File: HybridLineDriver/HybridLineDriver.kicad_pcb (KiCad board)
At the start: 2 copper layers, 100 x 50 mm, 60 parts, among them J1 XLR3, J2 Conn_01x03, J3 Conn_01x02, J4 XLR3, J5 Conn_01x02, U1 OPA1679, U2 OPA1679

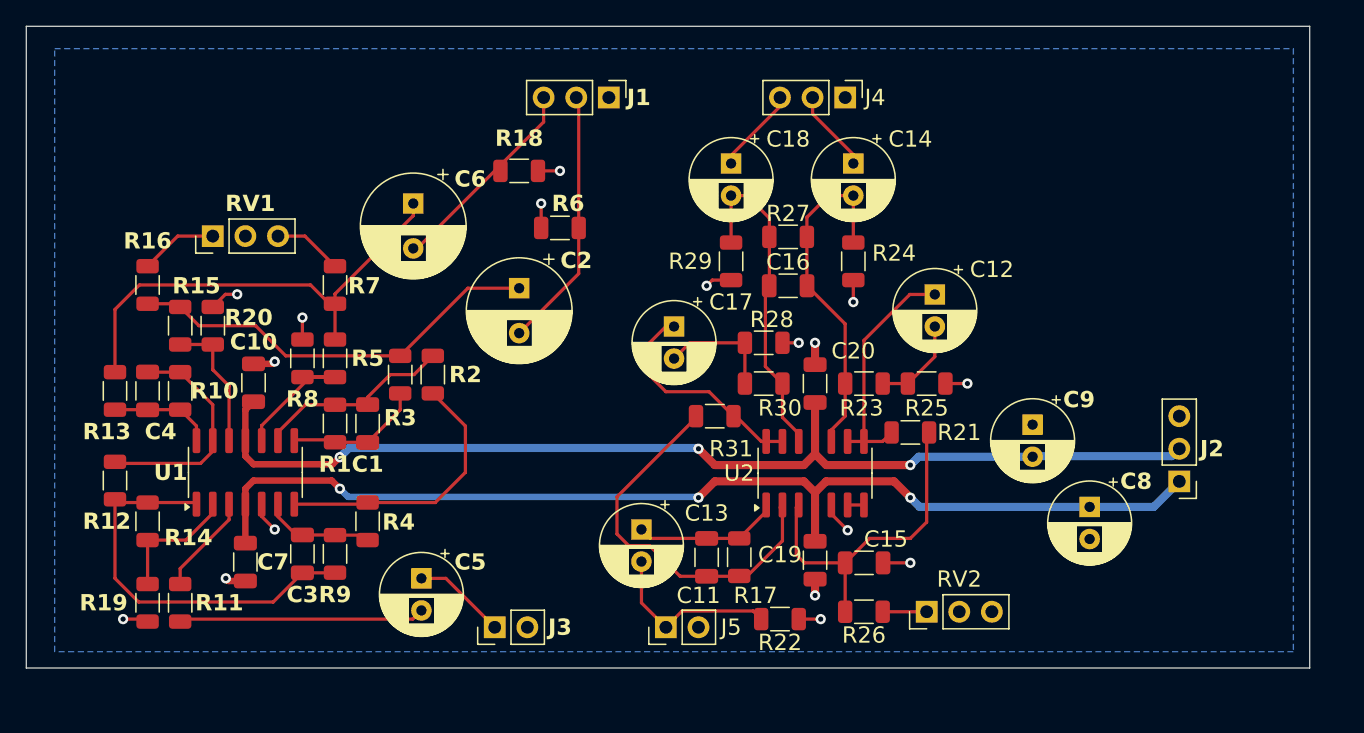
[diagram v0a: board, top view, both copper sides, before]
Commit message: added comments
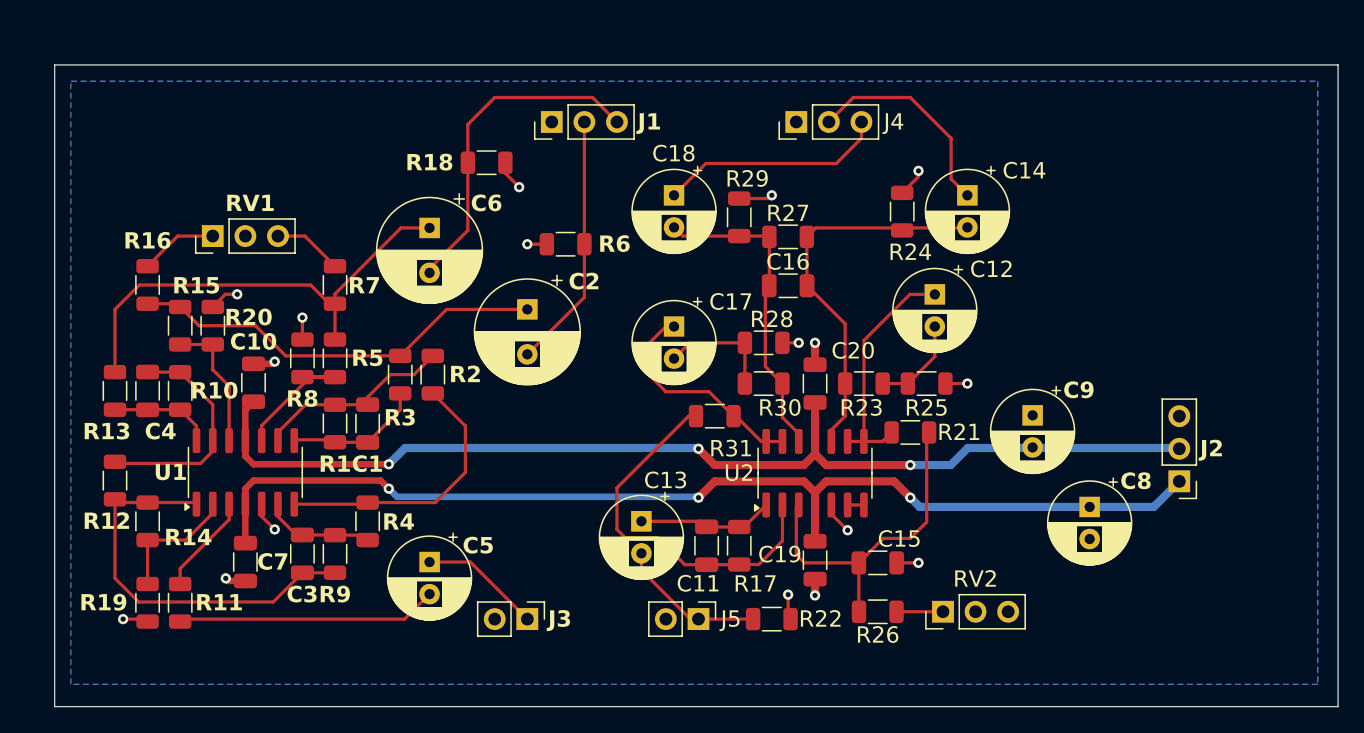
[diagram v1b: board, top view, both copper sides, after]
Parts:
- moved C14 9.23 mm to (114.3, 91.4)
- moved R24 5.43 mm to (109.2, 92.7), turned to -90 degrees
- moved C18 5.09 mm to (91.4, 91.4)
- moved J1 4.84 mm to (81.9, 85.7), turned to 90 degrees
- moved J4 4.26 mm to (101.0, 85.7), turned to 90 degrees
- moved R29 3.49 mm to (96.5, 93.2), turned to 90 degrees
- moved J3 2.62 mm to (80.0, 124.5), turned to -90 degrees
- moved R18 2.62 mm to (76.8, 88.9)
- moved J5 2.62 mm to (93.3, 124.5), turned to -90 degrees
- moved C6 2.29 mm to (72.4, 94.0)
- moved C2 1.77 mm to (80.0, 100.3)
- moved C5 1.42 mm to (72.4, 120.0)
- moved R6 1.34 mm to (83.0, 95.2)
- moved RV2 1.27 mm to (112.4, 123.9)
- moved R26 1.08 mm to (107.3, 123.9)
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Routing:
- net Net-(C18-Pad1): track 6.72 -> 17.7 mm
- net Net-(C14-Pad1): track 6.46 -> 16.6 mm
- net Net-(C6-Pad2): track 16.4 -> 26.1 mm
- net Net-(U2C-+): track 27.1 -> 30.4 mm
- net Net-(J5-Pin_1): track 14.1 -> 11.6 mm
- net Net-(J3-Pin_1): track 7.29 -> 9.46 mm
- net GND: track 32.0 -> 33.2 mm
- net Net-(C5-Pad2): track 19.2 -> 20.3 mm
- net Net-(U2D-+): track 26.0 -> 24.9 mm
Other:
- board text added: "GND"
- board text added: "IN"
- board text added: "IN+"
- board text added: "IN-"
- board text added: "OUT"
- board text added: "OUT+"
- board text added: "OUT-"
- board text added: "V+"
- board text added: "V-"
